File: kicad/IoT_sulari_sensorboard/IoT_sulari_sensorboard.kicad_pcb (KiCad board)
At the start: 2 copper layers, 8 parts, among them J1 20021121-00010C4LF, U1 SHT40-AD1B-R3, U2 TMP117MAIDRVT

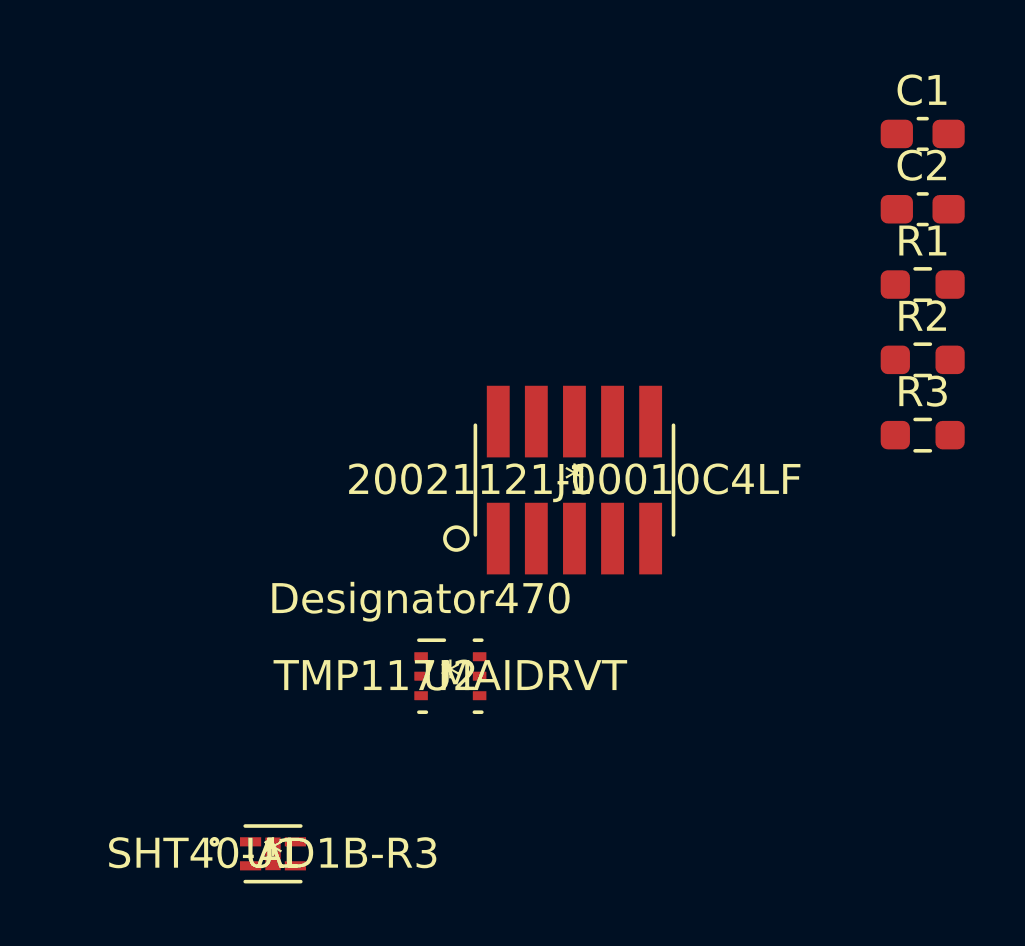
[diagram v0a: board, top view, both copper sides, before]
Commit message: sensorboard pcb drawing
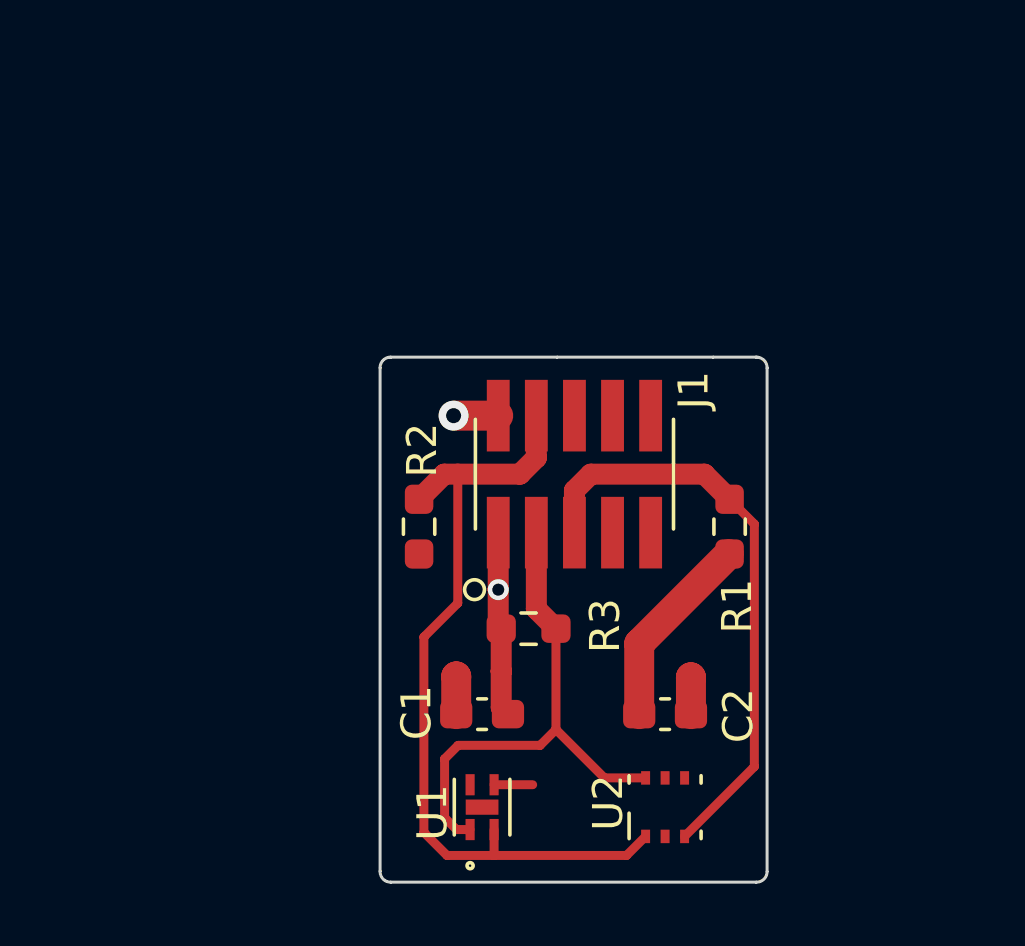
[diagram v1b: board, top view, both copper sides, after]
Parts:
- moved C1 24.3 mm to (135.0, 94.0), turned to 180 degrees
- moved C2 18.9 mm to (141.1, 94.0)
- moved R2 17.7 mm to (132.9, 87.8), turned to 90 degrees
- moved R3 14.6 mm to (136.6, 91.2)
- moved R1 10.3 mm to (143.2, 87.8), turned to 90 degrees
- moved U2 8.38 mm to (141.1, 97.1), turned to 90 degrees
- moved U1 7.14 mm to (135.0, 97.1), turned to 90 degrees
- moved J1 0.20 mm to (138.1, 86.0)
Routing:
- net /SCL: track 0.00 -> 27.1 mm
- net /TMP_ALERT: track 0.00 -> 19.7 mm
- net /SDA: track 0.00 -> 17.6 mm
- net /VCC: track 0.00 -> 14.1 mm, vias 0 -> 1
- net /GND: track 0.00 -> 3.98 mm, vias 0 -> 1
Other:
- board outline added: 12.9 x 17.5 mm
- rule pad_to_mask_clearance: 0 -> 0.05
